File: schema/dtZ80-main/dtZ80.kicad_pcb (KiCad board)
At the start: 2 copper layers, 121.9 x 67.3 mm, 9 parts, among them J1 PRPC040SAAN-RC, U1 Z80CPU, U2 28C256, U3 74LS32, X1 CXO_DIP8

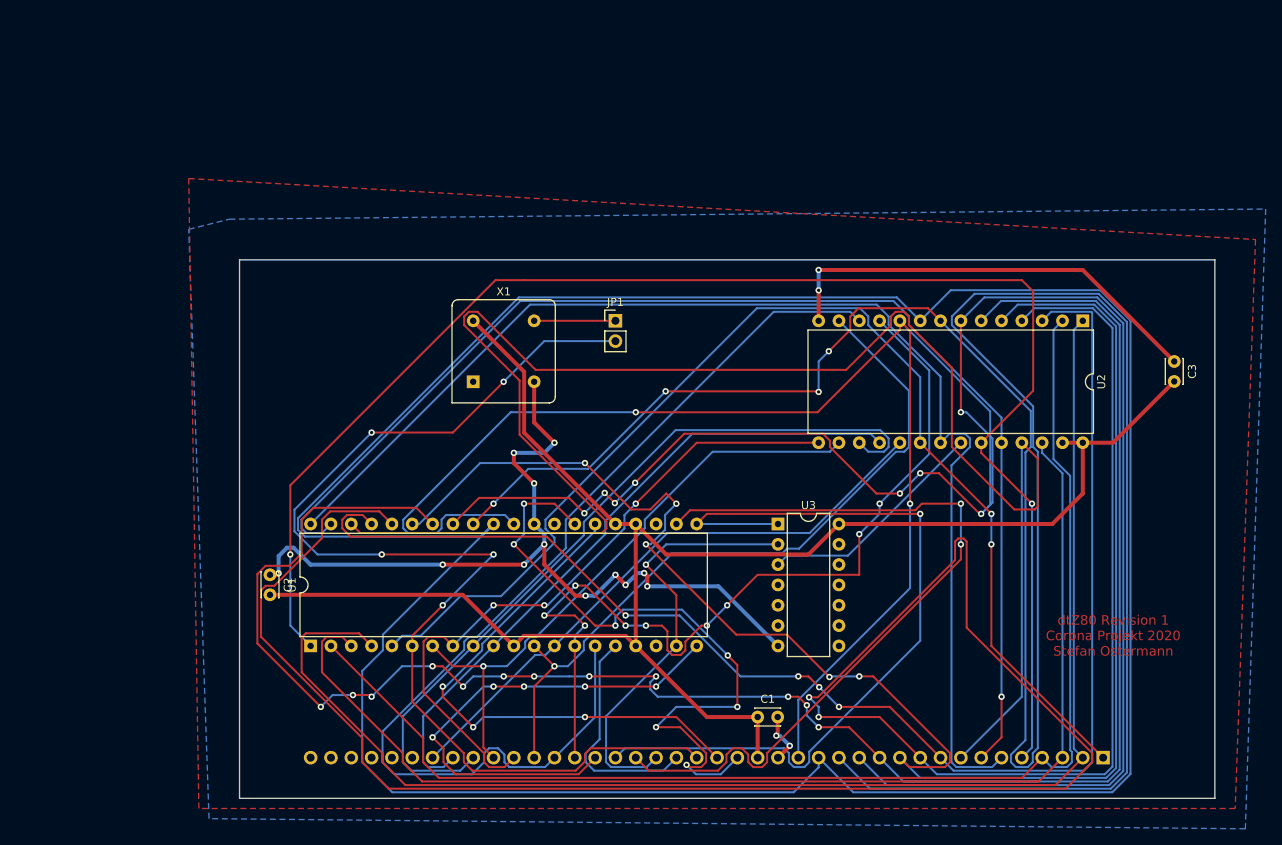
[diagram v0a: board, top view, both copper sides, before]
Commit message: Reworked Boards
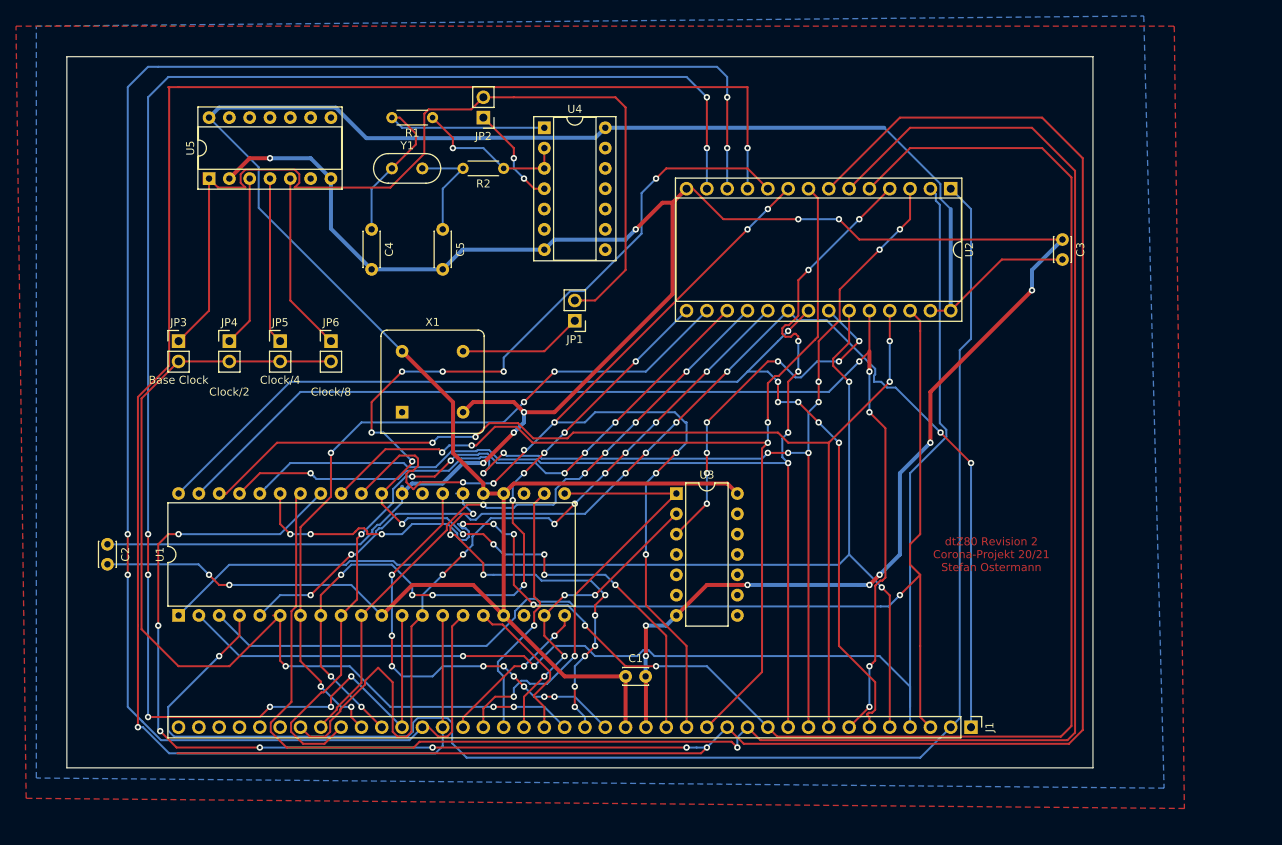
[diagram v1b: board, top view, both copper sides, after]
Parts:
- added C4: 22pF, Capacitor_THT:C_Disc_D4.3mm_W1.9mm_P5.00mm, F.Cu at (0.00, 45.7)
- added C5: 22pF, Capacitor_THT:C_Disc_D4.3mm_W1.9mm_P5.00mm, F.Cu at (8.89, 45.7)
- added JP2: Y1, Connector_PinHeader_2.54mm:PinHeader_1x02_P2.54mm_Vertical, F.Cu at (14.0, 31.8)
- added JP3: Base Clock, Connector_PinHeader_2.54mm:PinHeader_1x02_P2.54mm_Vertical, F.Cu at (-24.1, 59.7)
- added JP4: Clock/2, Connector_PinHeader_2.54mm:PinHeader_1x02_P2.54mm_Vertical, F.Cu at (-17.8, 59.7)
- added JP5: Clock/4, Connector_PinHeader_2.54mm:PinHeader_1x02_P2.54mm_Vertical, F.Cu at (-11.4, 59.7)
- added JP6: Clock/8, Connector_PinHeader_2.54mm:PinHeader_1x02_P2.54mm_Vertical, F.Cu at (-5.08, 59.7)
- added R1: 1M, Resistor_THT:R_Axial_DIN0204_L3.6mm_D1.6mm_P5.08mm_Horizontal, F.Cu at (7.62, 31.8)
- added R2: 1K, Resistor_THT:R_Axial_DIN0204_L3.6mm_D1.6mm_P5.08mm_Horizontal, F.Cu at (16.5, 38.1)
- added U4: 74LS04, Package_DIP:DIP-14_W7.62mm_Socket, F.Cu at (21.6, 33.0)
- added U5: 74LS393, Package_DIP:DIP-14_W7.62mm_Socket, F.Cu at (-20.3, 39.4)
- added Y1: Crystal, Crystal:Crystal_HC52-8mm_Vertical, F.Cu at (2.54, 38.1)
- J1: value PRPC040SAAN-RC -> RC2014Bus; moved to F.Cu
- JP1: value Jumper_2_Open -> X1
- U2: footprint Package_DIP:DIP-28_W15.24mm -> dtZ80-main:DIP-28_W15.24mm_Socket_Large_Holes
- moved U2 23.3 mm to (72.4, 40.6)
- moved C2 20.7 mm to (-33.0, 85.1)
- moved C3 20.7 mm to (86.4, 47.0)
- moved C1 17.3 mm to (31.8, 101.6)
- moved U1 16.9 mm to (-24.1, 94.0)
- moved J1 16.9 mm to (74.9, 108.0), turned to 270 degrees
- moved U3 13.3 mm to (38.1, 78.7)
- moved X1 9.67 mm to (3.81, 68.6)
- moved JP1 5.08 mm to (25.4, 57.1), turned to 180 degrees
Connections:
- J1 pad 35: Net-(J1-Pad35) -> (no net)
- J1 pad 36: Net-(J1-Pad36) -> (no net)
- J1 pad 37: Net-(J1-Pad37) -> (no net)
- J1 pad 38: Net-(J1-Pad38) -> (no net)
- J1 pad 39: Net-(J1-Pad39) -> (no net)
- J1 pad 40: Net-(J1-Pad40) -> (no net)
- JP1 pad 2: /CLK -> /CLK_BASE
- U1 pad 18: Net-(U1-Pad18) -> (no net)
- U1 pad 23: Net-(U1-Pad23) -> (no net)
- U1 pad 28: Net-(U1-Pad28) -> (no net)
- X1 pad 1: Net-(X1-Pad1) -> (no net)
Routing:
- net /A1: track 342.8 -> 136.8 mm, vias 0 -> 9
- net /A2: track 317.3 -> 131.8 mm
- net /A6: track 317.6 -> 145.7 mm, vias 2 -> 6
- net GND: track 168.5 -> 323.5 mm, vias 16 -> 14
- net /D2: track 91.8 -> 212.1 mm, vias 1 -> 8
- net /CLK_BASE: track 0.00 -> 116.3 mm
- net +5V: track 208.1 -> 323.4 mm, vias 0 -> 2
- net /D0: track 111.3 -> 223.9 mm, vias 9 -> 2
- net /D1: track 130.5 -> 227.4 mm, vias 0 -> 5
- net /A3: track 248.9 -> 340.8 mm, vias 8 -> 7
- net /A8: track 213.2 -> 136.7 mm, vias 0 -> 4
- net /WR: track 99.5 -> 32.5 mm, vias 2 -> 1
- net /A11: track 189.3 -> 143.2 mm
- net /RD: track 102.0 -> 57.0 mm, vias 1 -> 2
- net /IORQ: track 61.9 -> 19.9 mm, vias 5 -> 2
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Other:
- board size 121.9 x 67.3 mm -> 128.3 x 88.9 mm
- board text added: "dtZ80 Revision 2 Corona-Projekt 20/21 Stefan Ostermann"
- board text removed: "dtZ80 Revision 1 Corona Projekt 2020 Stefan Ostermann"
